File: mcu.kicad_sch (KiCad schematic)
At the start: 1 part, among them U7 ADA3708

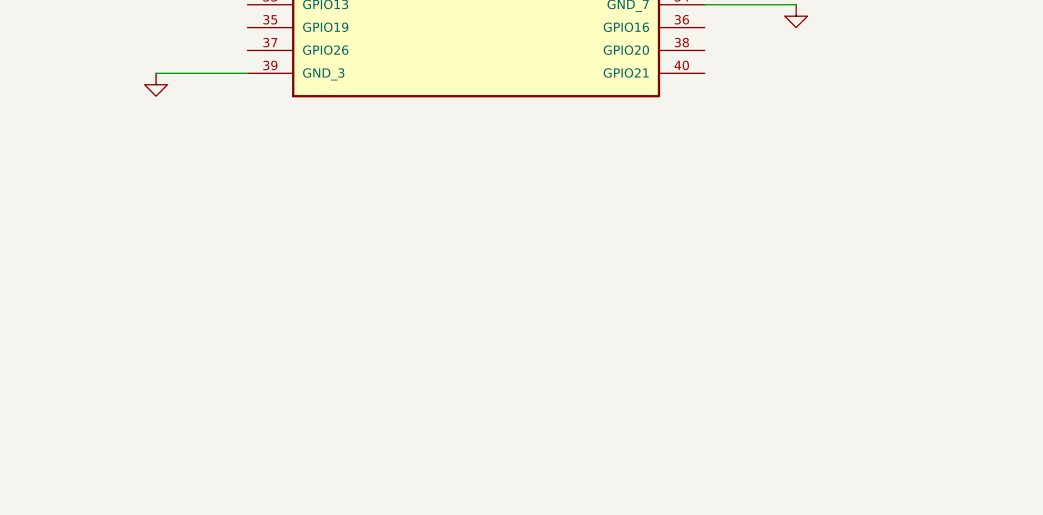
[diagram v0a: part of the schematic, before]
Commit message: gps started
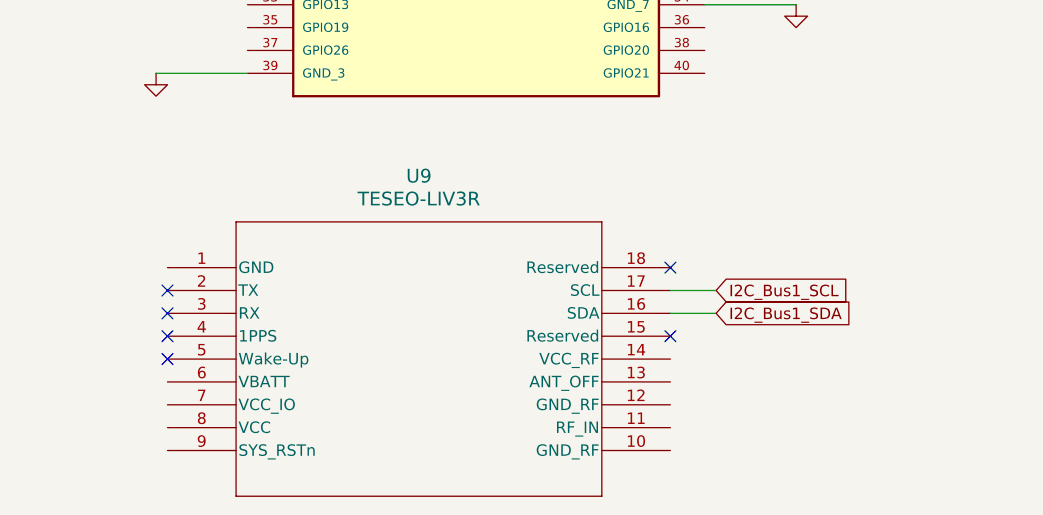
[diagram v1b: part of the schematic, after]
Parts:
- added U9: TESEO-LIV3R, ARRAY_LIV3R_STM, symbol Teseo Liver:TESEO-LIV3R
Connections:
- net I2C_Bus1_SCL: now also U9.17 (SCL)
- net I2C_Bus1_SDA: now also U9.16 (SDA)
- no-connect marks 0 -> 6
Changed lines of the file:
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@@
 (kicad_sch (version 20230121) (generator eeschema)
   (paper "A4")
+  (no_connect (at 118.11 140.97))
+  (no_connect (at 118.11 143.51))
+  (no_connect (at 118.11 146.05))
+  (no_connect (at 173.99 146.05))
+  (no_connect (at 173.99 138.43))
+  (no_connect (at 118.11 148.59))
   (wire (pts (xy 187.96 109.22) (xy 177.8 109.22))
     (stroke (width 0) (type default))
   )
+  (wire (pts (xy 179.07 143.51) (xy 173.99 143.51))
+    (stroke (width 0) (type default))
+  )
   (wire (pts (xy 116.84 116.84) (xy 127 116.84))
+    (stroke (width 0) (type default))
+  )
+  (wire (pts (xy 179.07 140.97) (xy 173.99 140.97))
     (stroke (width 0) (type default))
   )
@@
     (effects (font (size 1.27 1.27)) (justify left))
     (property "Intersheetrefs" "${INTERSHEET_REFS}" (at 223.1598 106.68 0)
+      (effects (font (size 1.27 1.27)) (justify left) hide)
+    )
+  )
+  (global_label "I2C_Bus1_SDA" (shape input) (at 179.07 143.51 0) (fields_autoplaced)
+    (effects (font (size 1.27 1.27)) (justify left))
+    (property "Intersheetrefs" "${INTERSHEET_REFS}" (at 195.22 143.51 0)
+      (effects (font (size 1.27 1.27)) (justify left) hide)
+    )
+  )
+  (global_label "I2C_Bus1_SCL" (shape input) (at 179.07 140.97 0) (fields_autoplaced)
+    (effects (font (size 1.27 1.27)) (justify left))
+    (property "Intersheetrefs" "${INTERSHEET_REFS}" (at 195.1595 140.97 0)
       (effects (font (size 1.27 1.27)) (justify left) hide)
     )
@@
         )
       )
+    )
+  )
+  (symbol (lib_id "Teseo Liver:TESEO-LIV3R") (at 118.11 138.43 0) (unit 1)
+    (in_bom yes) (on_board yes) (dnp no) (fields_autoplaced)
+    (property "Reference" "U9" (at 146.05 128.27 0)
+      (effects (font (size 1.524 1.524)))
+    )
+    (property "Value" "TESEO-LIV3R" (at 146.05 130.81 0)
+      (effects (font (size 1.524 1.524)))
+    )
+    (property "Footprint" "ARRAY_LIV3R_STM" (at 118.11 138.43 0)
+      (effects (font (size 1.27 1.27) italic) hide)
+    )
+    (property "Datasheet" "TESEO-LIV3R" (at 118.11 138.43 0)
+      (effects (font (size 1.27 1.27) italic) hide)
+    )
+    (pin "1")
+    (pin "10")
+    (pin "11")
+    (pin "12")
+    (pin "13")
+    (pin "14")
+    (pin "15")
+    (pin "16")
+    (pin "17")
+    (pin "18")
+    (pin "2")
+    (pin "3")
+    (pin "4")
+    (pin "5")
+    (pin "6")
+    (pin "7")
+    (pin "8")
+    (pin "9")
+    (instances
+      (project "Watersphere mobo"
+        (path "/c4a63ad0-0af5-4f61-bde7-7fb53fc8413c/3f8884fe-4665-4fba-a6c0-e9032b67a8f5"
+          (reference "U9") (unit 1)
+        )
+      )
